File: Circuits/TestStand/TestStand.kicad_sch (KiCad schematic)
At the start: 2 parts, among them U1 INA125UA

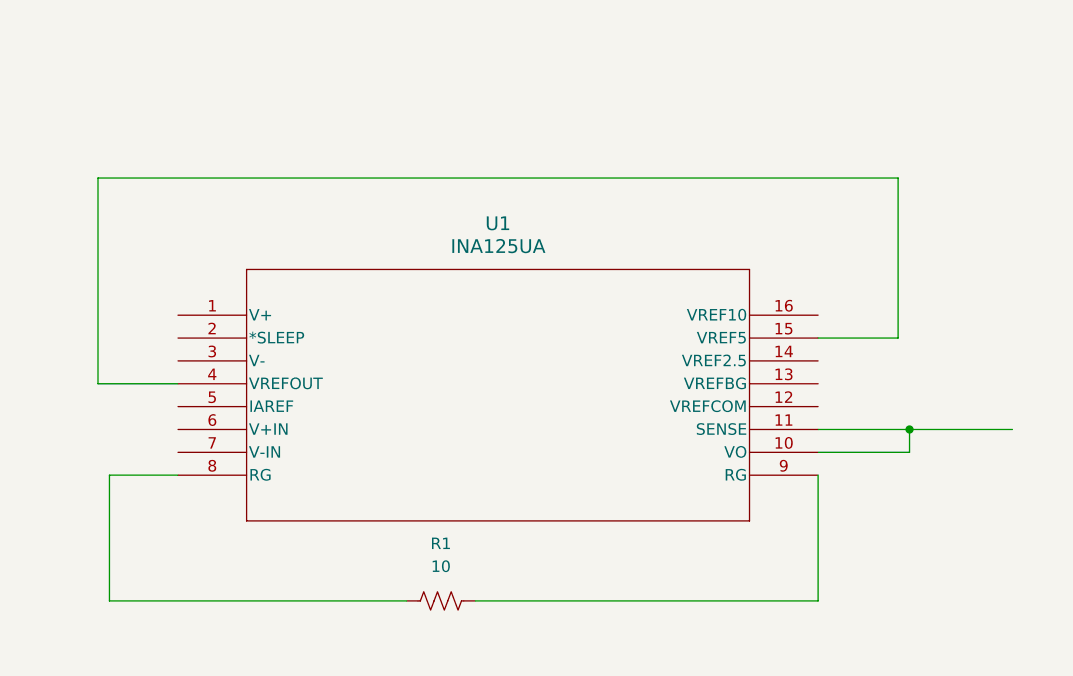
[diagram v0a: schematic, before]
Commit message: HX711 Load Cell Circuitry
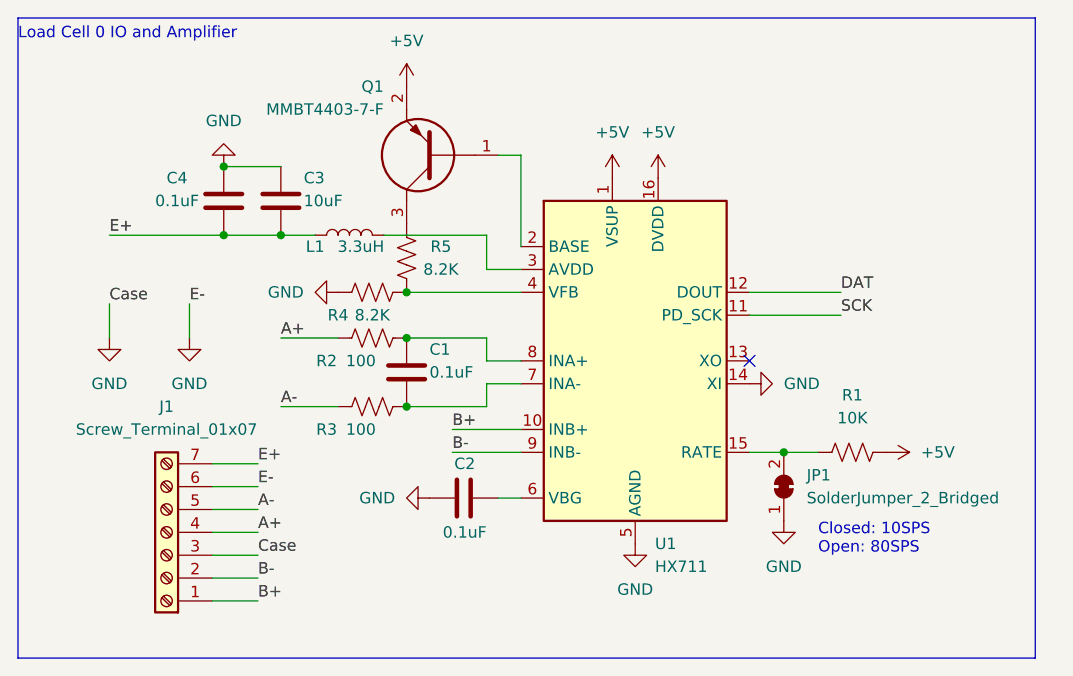
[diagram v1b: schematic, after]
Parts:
- removed U1: INA125UA, D16, symbol 2024-08-07_02-08-08:INA125UA
- added C1, C2, C4: 0.1uF, symbol Device:C
- added C3: 10uF, symbol Device:C
- added J1: Screw_Terminal_01x07, symbol Connector:Screw_Terminal_01x07
- added JP1: SolderJumper_2_Bridged, symbol Jumper:SolderJumper_2_Bridged
- added L1: 3.3uH, symbol Device:L
- added Q1: MMBT4403-7-F, SOT96P240X110-3N, symbol MMBT4403-7-F:MMBT4403-7-F
- added R2, R3: 100, symbol Device:R_US
- added R4, R5: 8.2K, symbol Device:R_US
- added U1: HX711, Package_SO:SOP-16_3.9x9.9mm_P1.27mm, symbol Analog_ADC:HX711
- R1: value 10 -> 10K
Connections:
- net at R1.1: now also JP1.2 (B), U1.15 (RATE)
- net +5V: now reaches R1.2
- net +5V: now also Q1.2, U1.1 (VSUP), U1.16 (DVDD)
- new net: C1.1, R3.2, U1.7 (INA-)
- new net: C1.2, R2.2, U1.8 (INA+)
- new net: L1.2, U1.3 (AVDD)
- new net: Q1.1, U1.2 (BASE)
- new net: Q1.3, R5.1
- new net: R4.2, R5.2, U1.4 (VFB)
- new net: C2.1, U1.6 (VBG)
- new net A+: J1.4 (Pin_4), R2.1
- new net A-: J1.5 (Pin_5), R3.1
- new net B+: J1.1 (Pin_1), U1.10 (INB+)
- new net B-: J1.2 (Pin_2), U1.9 (INB-)
- new net DAT: U1.12 (DOUT)
- new net E+: C3.1, C4.1, J1.7 (Pin_7), L1.1
- new net GND: C2.2, C3.2, C4.2, J1.3 (Pin_3), J1.6 (Pin_6), JP1.1 (A), R4.1, U1.14 (XI), U1.5 (AGND)
- new net SCK: U1.11 (PD_SCK)
- no-connect marks 0 -> 1
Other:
- note added: "Closed: 10SPS Open: 80SPS"
- note added: "Load Cell 0 IO and Amplifier"
